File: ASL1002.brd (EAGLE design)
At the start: 12.8 x 6.5 mm, 5 parts

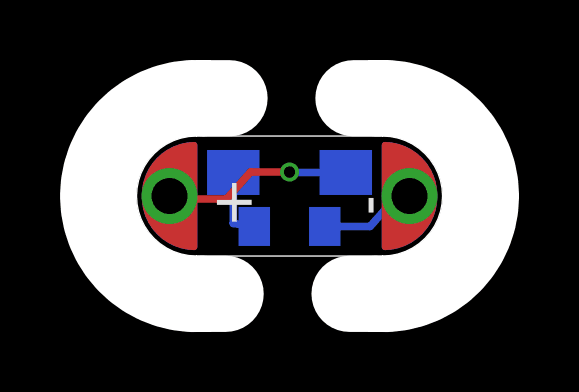
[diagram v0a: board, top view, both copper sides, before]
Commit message: Updated to Rev 2
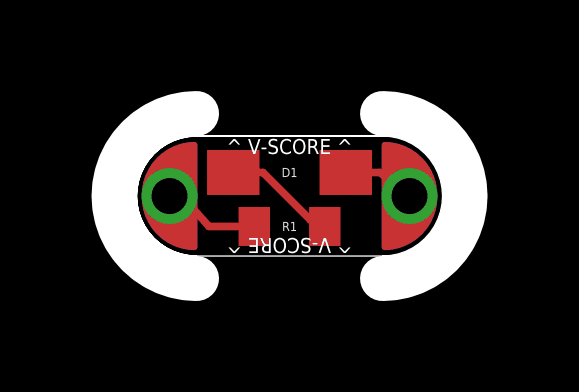
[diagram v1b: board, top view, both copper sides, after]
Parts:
- moved U$1 8.00 mm to (16.0, 20.0), flipped to the bottom
- moved U$7 8.00 mm to (24.0, 20.0), flipped to the bottom
- flipped D1 to the top, turned to 180 degrees
- flipped R1 to the top
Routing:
- net +: track 6.32 -> 2.40 mm, vias 1 -> 0
- net N$2: track 2.41 -> 3.86 mm
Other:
- board size 12.8 x 6.5 mm -> 11.7 x 5.5 mm
- board text added: "2"
- board text added: "^ V-SCORE ^"
- board text removed: "1"
